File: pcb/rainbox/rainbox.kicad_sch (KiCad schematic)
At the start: 14 parts, among them J1 USB_C_Receptacle_USB2.0_14P, J2 Conn_01x04_Pin, U1 ESP32-S3-WROOM-2, U2 LM3940IMPX-3.3/NOPB, U3 ESC, U4 TMC2240_Module

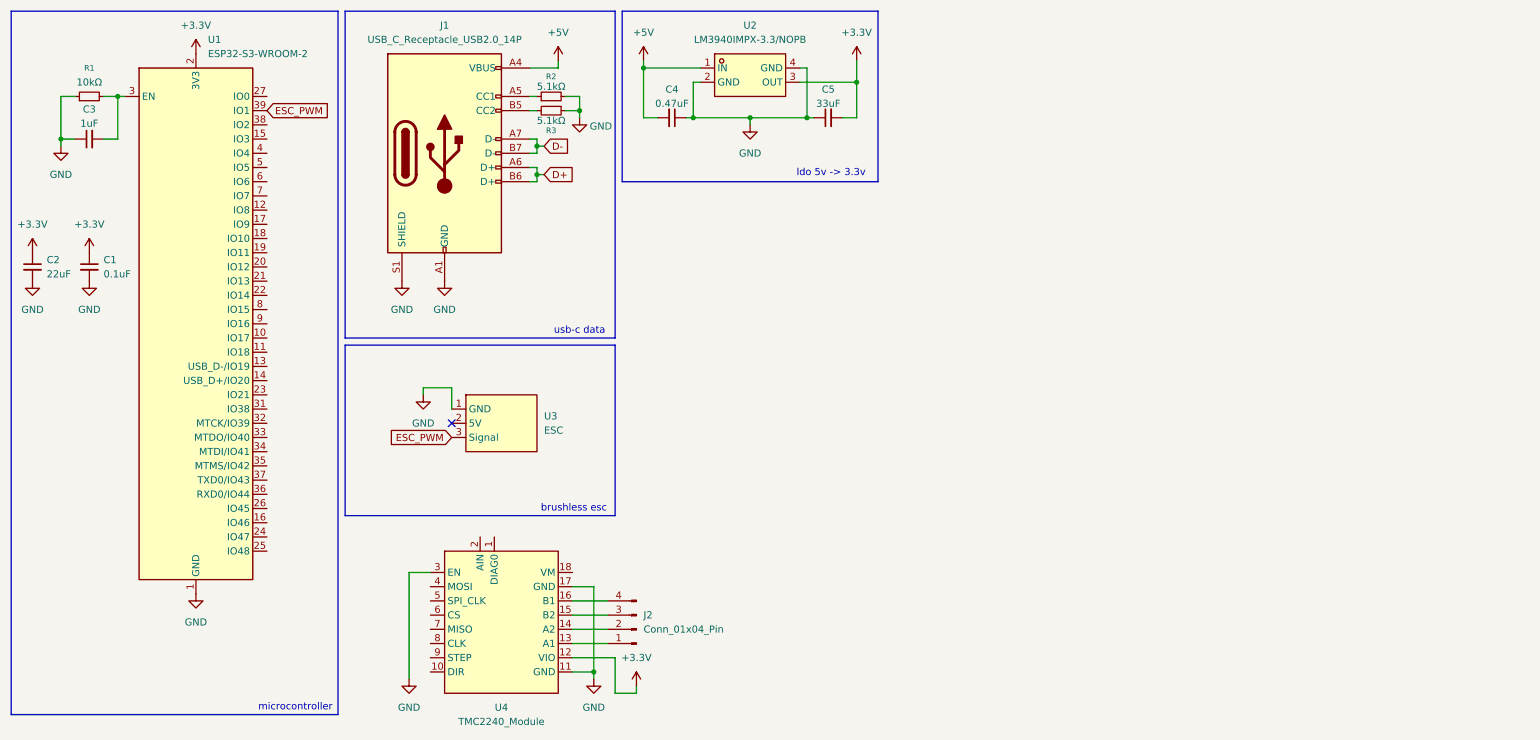
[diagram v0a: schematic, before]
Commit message: more kicad additions and research
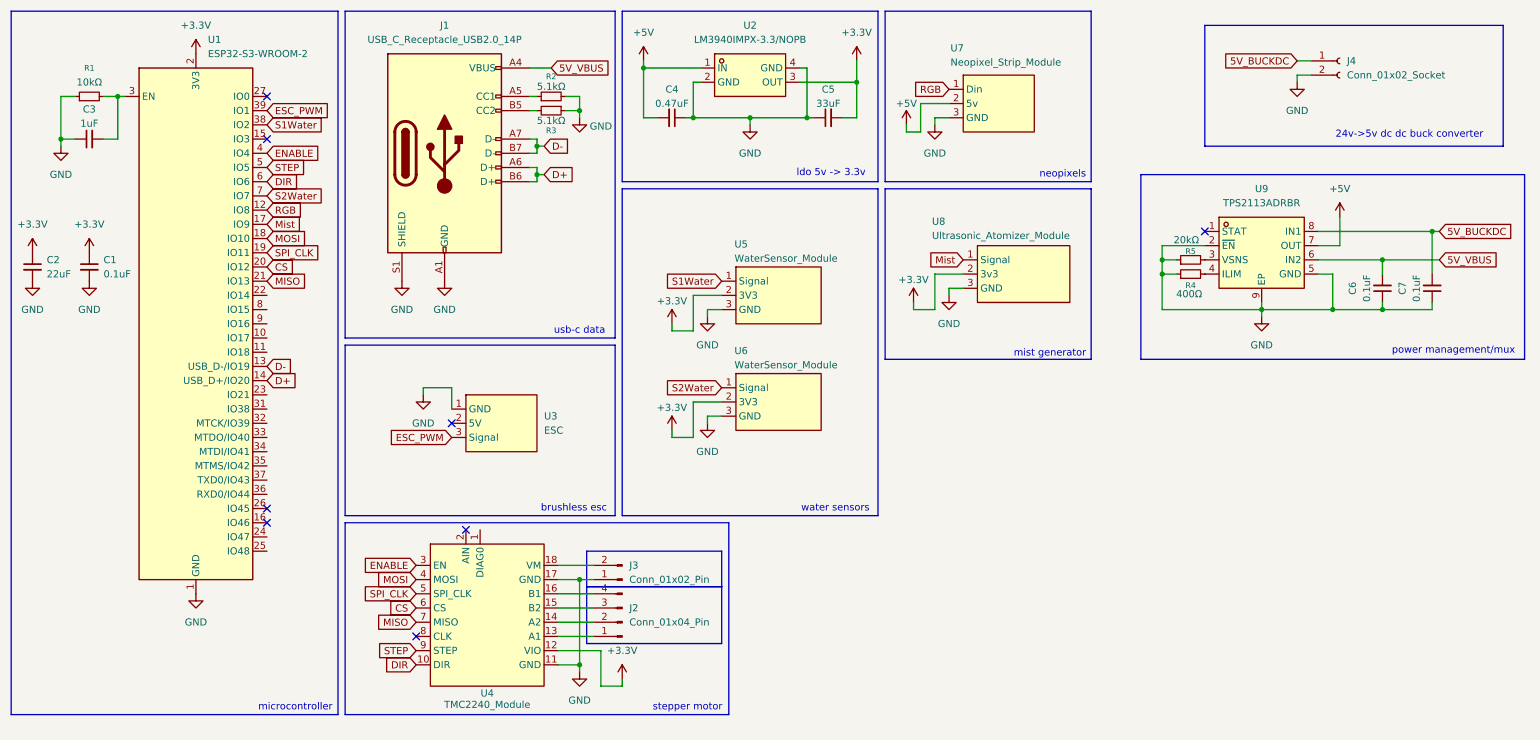
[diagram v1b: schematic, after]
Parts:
- added C6, C7: 0.1uF, symbol Device:C_Small
- added J3: Conn_01x02_Pin, symbol Connector:Conn_01x02_Pin
- added J4: Conn_01x02_Socket, Connector_PinSocket_2.54mm:PinSocket_1x02_P2.54mm_Vertical, symbol Connector:Conn_01x02_Socket
- added R4: 400Ω, symbol Device:R_Small
- added R5: 20kΩ, symbol Device:R_Small
- added U5, U6: WaterSensor_Module, Connector_PinHeader_2.54mm:PinHeader_1x03_P2.54mm_Vertical, symbol 1_udu_lib:Water_Sensor_Module
- added U7: Neopixel_Strip_Module, Connector_PinHeader_2.54mm:PinHeader_1x03_P2.54mm_Vertical, symbol 1_udu_lib:Neopixel_Strip_Module
- added U8: Ultrasonic_Atomizer_Module, Connector_PinHeader_2.54mm:PinHeader_1x03_P2.54mm_Vertical, symbol 1_udu_lib:Ultrasonic_Atomizer_Module
- added U9: TPS2113ADRBR, EasyEDA:SON-8_L3.0-W3.0-P0.65-LS3.0-BL-EP, symbol EasyEDA:TPS2113ADRBR
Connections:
- net +3.3V: now also U5.2 (3V3), U6.2 (3V3), U8.2 (3v3)
- net +5V: now also U7.2 (5v), U9.7 (OUT); no longer J1.A4 (VBUS), J1.A9 (VBUS), J1.B4 (VBUS), J1.B9 (VBUS)
- net D+: now also U1.14 (USB_D+/IO20)
- net D-: now also U1.13 (USB_D-/IO19)
- net GND: now also C6.1, C7.1, J3.1 (Pin_1), J4.2 (Pin_2), R4.1, R5.1, U5.3 (GND), U6.3 (GND), U7.3 (GND), U8.3 (GND), U9.2 (~{EN}), U9.5 (GND), U9.9 (EP); no longer U4.3 (EN)
- net DIR: now reaches U4.10 (DIR)
- net DIR: now also U1.6 (IO6)
- net at U4.18 (VM): now also J3.2 (Pin_2)
- net MOSI: now reaches U4.4 (MOSI)
- net MOSI: now also U1.18 (IO10)
- net SPI_CLK: now reaches U4.5 (SPI_CLK)
- net SPI_CLK: now also U1.19 (IO11)
- net CS: now reaches U4.6 (CS)
- net CS: now also U1.20 (IO12)
- net MISO: now reaches U4.7 (MISO)
- net MISO: now also U1.21 (IO13)
- net STEP: now reaches U4.9 (STEP)
- net STEP: now also U1.5 (IO5)
- net RGB: now reaches U1.12 (IO8)
- net RGB: now also U7.1 (Din)
- net Mist: now reaches U1.17 (IO9)
- net Mist: now also U8.1 (Signal)
- net S1Water: now reaches U1.38 (IO2)
- net S1Water: now also U5.1 (Signal)
- net ENABLE: now reaches U1.4 (IO4)
- net ENABLE: now also U4.3 (EN)
- net S2Water: now reaches U1.7 (IO7)
- net S2Water: now also U6.1 (Signal)
- new net: R4.2, U9.4 (ILIM)
- new net: R5.2, U9.3 (VSNS)
- new net 5V_BUCKDC: C7.2, J4.1 (Pin_1), U9.8 (IN1)
- new net 5V_VBUS: C6.2, J1.A4 (VBUS), J1.A9 (VBUS), J1.B4 (VBUS), J1.B9 (VBUS), U9.6 (IN2)
- no-connect marks 1 -> 8
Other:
- note added: "24v->5v dc dc buck converter"
- note added: "mist generator"
- note added: "neopixels"
- note added: "power management/mux"
- note added: "stepper motor"
- note added: "water sensors"
- moved on the sheet: J2
